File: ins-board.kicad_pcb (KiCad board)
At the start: 4 copper layers, 50 x 23 mm, 94 parts, among them P1 PWR, P2 Power (Solder Pad), Q1 FDN306P, Q2 FDC638APZ, U1 24LC128, U10 HMC5883L, U11 H3LIS331DL, U2 STM32F415RGT6, U3 LTC4412, U4 MAX3051, U5 LT1965, U6 LT1761-3.3, U7 LT1965, U8 MS5611-01BA, U9 MPU6000, X1 CRYSTAL 16MHz 10ppm

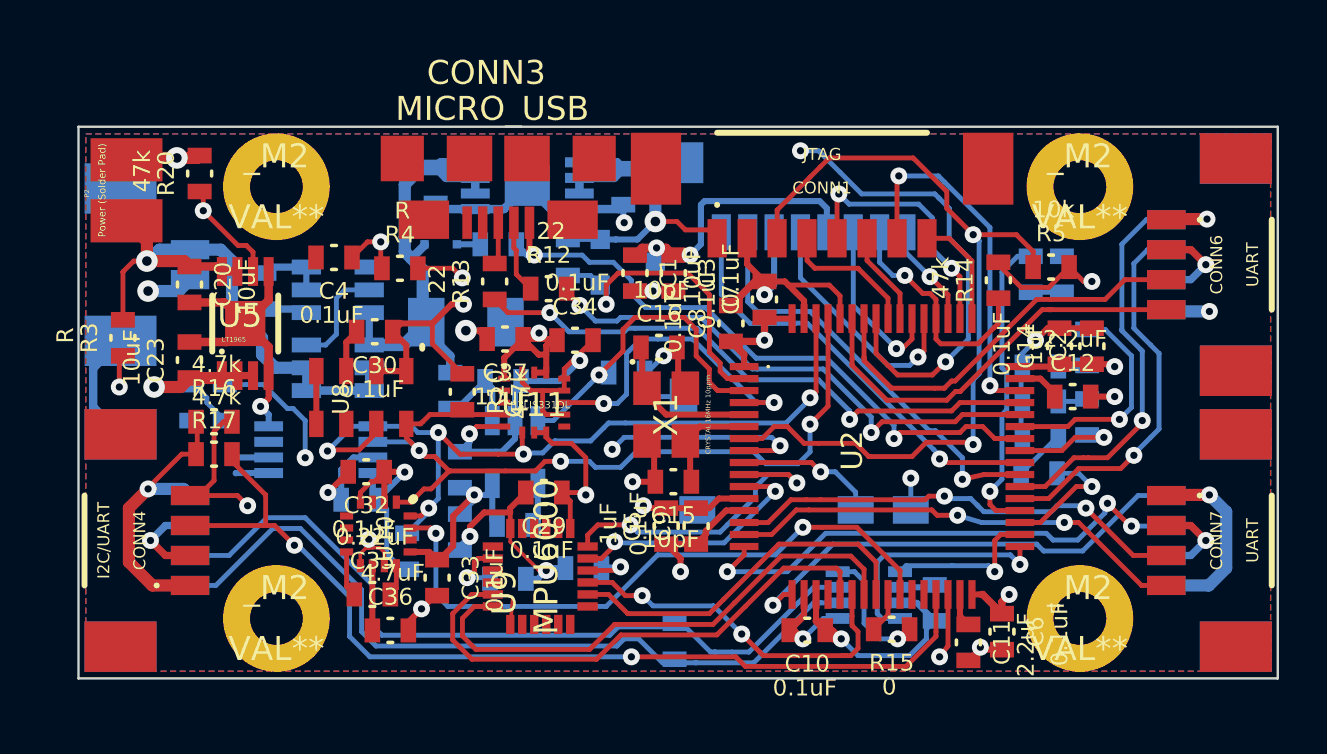
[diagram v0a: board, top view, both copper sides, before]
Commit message: optimize routing
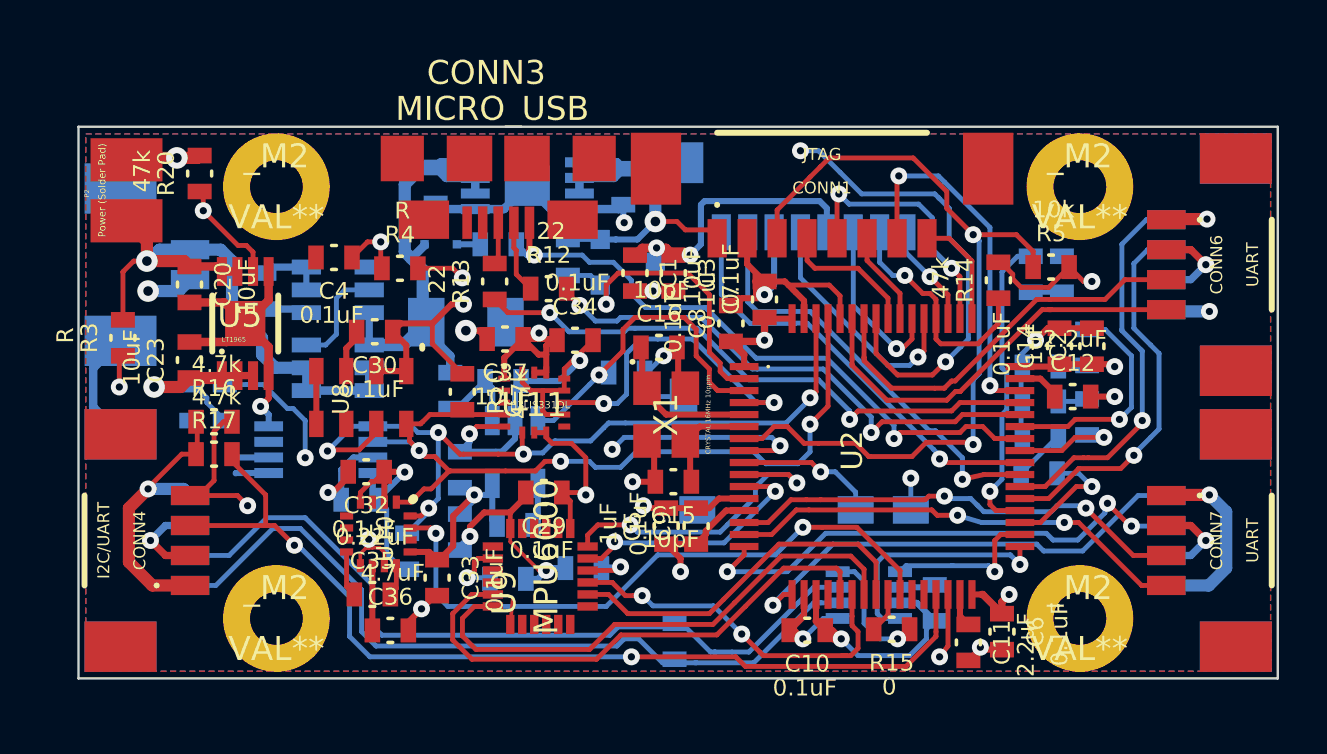
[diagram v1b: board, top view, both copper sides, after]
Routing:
- net GND: track 143.3 -> 144.7 mm
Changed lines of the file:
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@@
     (thickness 1.6)
     (drawings 13)
-    (tracks 1282)
+    (tracks 1293)
     (zones 0)
     (modules 94)
@@
   )
   (setup
-    (last_trace_width 0.2032)
+    (last_trace_width 0.254)
     (user_trace_width 0.1524)
     (user_trace_width 0.2032)
@@
   (segment (start 61.05 43.85) (end 56.15 43.85) (width 0.2032) (layer B.Cu) (net 27))
   (segment (start 62.2 42.7) (end 61.05 43.85) (width 0.2032) (layer B.Cu) (net 27))
-  (segment (start 45.6646 38.3872) (end 45.6646 38.9646) (width 0.2032) (layer F.Cu) (net 28))
-  (segment (start 45.6646 38.9646) (end 46.2 39.5) (width 0.2032) (layer F.Cu) (net 28))
+  (segment (start 45.6646 38.3872) (end 45.8 38.5226) (width 0.2032) (layer F.Cu) (net 28))
+  (segment (start 45.8 38.5226) (end 45.8 39.1) (width 0.2032) (layer F.Cu) (net 28))
+  (segment (start 45.8 39.1) (end 46.2 39.5) (width 0.2032) (layer F.Cu) (net 28))
   (segment (start 46.85 39.75) (end 46.45 39.75) (width 0.2032) (layer F.Cu) (net 28))
   (segment (start 46.45 39.75) (end 46.2 39.5) (width 0.2032) (layer F.Cu) (net 28))
@@
   (segment (start 66.25 38.75) (end 66 39) (width 0.2032) (layer F.Cu) (net 51))
   (segment (start 66.25 38.75) (end 66 39) (width 0.2032) (layer F.Cu) (net 51))
+  (segment (start 60.6 33) (end 60.45 33.15) (width 0.254) (layer F.Cu) (net 52))
+  (segment (start 59.5 33.15) (end 59.2 33.45) (width 0.254) (layer F.Cu) (net 52) (status C00000))
+  (segment (start 59.7 33.15) (end 59.5 33.15) (width 0.254) (layer F.Cu) (net 52) (status C00000))
+  (segment (start 60.45 33.15) (end 59.7 33.15) (width 0.254) (layer F.Cu) (net 52) (status 800000))
+  (segment (start 60.6 32.45) (end 60.25 32.8) (width 0.254) (layer F.Cu) (net 52) (status 400000))
+  (segment (start 60.25 32.8) (end 60.25 33) (width 0.254) (layer F.Cu) (net 52))
+  (segment (start 60.25 33) (end 60.6 33) (width 0.254) (layer F.Cu) (net 52))
+  (segment (start 50.65 41.25) (end 50.65 41.42) (width 0.254) (layer F.Cu) (net 52) (status C00000))
+  (segment (start 50.65 41.42) (end 49.99 42.08) (width 0.254) (layer F.Cu) (net 52) (status 400000))
+  (segment (start 43.2428 40.386) (end 43.2428 40.6072) (width 0.254) (layer F.Cu) (net 52))
+  (segment (start 42.6 41.25) (end 42.4 41.25) (width 0.254) (layer F.Cu) (net 52))
+  (segment (start 43.2428 40.6072) (end 42.6 41.25) (width 0.254) (layer F.Cu) (net 52))
+  (segment (start 43.5984 34.544) (end 43.5984 34.8016) (width 0.254) (layer F.Cu) (net 52))
+  (segment (start 43.5984 34.8016) (end 43.1646 35.2354) (width 0.254) (layer F.Cu) (net 52))
   (segment (start 79 43.25) (end 79.65 43.25) (width 0.508) (layer Inner2.Cu) (net 52))
   (segment (start 46.15 31.9) (end 47.6 31.9) (width 0.2032) (layer F.Cu) (net 52))
@@
   (via (at 39.59 37.66) (size 0.706) (layers F.Cu B.Cu) (net 52))
   (segment (start 39.925 37.325) (end 39.59 37.66) (width 0.254) (layer F.Cu) (net 52))
-  (segment (start 49.99 42.08) (end 49.99 41.91) (width 0.254) (layer F.Cu) (net 52))
-  (segment (start 49.99 41.91) (end 50.65 41.25) (width 0.254) (layer F.Cu) (net 52))
   (segment (start 47.9 43.65) (end 47.9 43.5) (width 0.254) (layer B.Cu) (net 52))
   (segment (start 48.91 42.08) (end 49.99 42.08) (width 0.254) (layer F.Cu) (net 52))
@@
   (segment (start 50 42.75) (end 50 42.08) (width 0.2032) (layer F.Cu) (net 52))
   (segment (start 47.9 39.55) (end 49.4 39.55) (width 0.254) (layer B.Cu) (net 52))
-  (segment (start 43.2428 40.386) (end 43.2428 40.4072) (width 0.254) (layer F.Cu) (net 52))
-  (segment (start 43.2428 40.4072) (end 42.4 41.25) (width 0.254) (layer F.Cu) (net 52))
   (segment (start 42.4 41.25) (end 42.65 41.25) (width 0.2032) (layer B.Cu) (net 52))
   (via (at 42.4 41.25) (size 0.706) (layers F.Cu B.Cu) (net 52))
@@
   (segment (start 42.95 40.3) (end 43.4632 39.7868) (width 0.254) (layer B.Cu) (net 52))
   (segment (start 41.9146 38.3872) (end 41.9146 36.1872) (width 0.254) (layer F.Cu) (net 52))
-  (segment (start 43.1646 36.1872) (end 43.1646 34.9778) (width 0.254) (layer F.Cu) (net 52))
-  (segment (start 43.1646 34.9778) (end 43.5984 34.544) (width 0.254) (layer F.Cu) (net 52))
+  (segment (start 43.1646 36.1872) (end 43.1646 35.2354) (width 0.254) (layer F.Cu) (net 52))
   (segment (start 66.7 41.975) (end 66.7 40.65) (width 0.2032) (layer B.Cu) (net 52))
   (via (at 66.7 40.65) (size 0.706) (layers F.Cu B.Cu) (net 52))
@@
   (via (at 55.1 40.8) (size 0.706) (layers F.Cu B.Cu) (net 52))
   (segment (start 61 30.4) (end 61 32.6) (width 0.254) (layer B.Cu) (net 52))
+  (segment (start 61 32.6) (end 60.6 33) (width 0.254) (layer B.Cu) (net 52))
   (via (at 60.6 33) (size 0.706) (layers F.Cu B.Cu) (net 52))
   (segment (start 60.6 33) (end 60.6 32.45) (width 0.254) (layer F.Cu) (net 52))
-  (segment (start 61 32.6) (end 60.6 33) (width 0.254) (layer B.Cu) (net 52))
   (segment (start 66.25 45.2) (end 67.6 45.2) (width 0.254) (layer B.Cu) (net 52))
   (segment (start 67.6 45.2) (end 67.7 45.1) (width 0.254) (layer B.Cu) (net 52))
@@
   (segment (start 61.6 32.6) (end 61.45 32.45) (width 0.254) (layer F.Cu) (net 52))
   (segment (start 61.45 32.45) (end 60.2 32.45) (width 0.254) (layer F.Cu) (net 52))
-  (segment (start 60.2 32.45) (end 59.2 33.45) (width 0.3048) (layer F.Cu) (net 52))
   (segment (start 77.35 31.125) (end 78.375 31.125) (width 0.3048) (layer F.Cu) (net 52))
   (segment (start 78.375 32.375) (end 77.35 32.375) (width 0.3048) (layer B.Cu) (net 52))
@@
   (via (at 54.6 44.35) (size 0.706) (layers F.Cu B.Cu) (net 76))
   (segment (start 54.45 44.5) (end 54.6 44.35) (width 0.2032) (layer F.Cu) (net 76))
+  (segment (start 70.35 31.65) (end 70.45 31.65) (width 0.2032) (layer F.Cu) (net 77) (status C00000))
+  (segment (start 70.95 32.15) (end 70.95 32.35) (width 0.2032) (layer F.Cu) (net 77))
+  (segment (start 70.45 31.65) (end 70.95 32.15) (width 0.2032) (layer F.Cu) (net 77) (status 400000))
   (segment (start 44.275 30.175) (end 45.6 28.85) (width 0.2032) (layer Inner2.Cu) (net 77))
   (segment (start 45.6 28.85) (end 54.05 28.85) (width 0.2032) (layer Inner2.Cu) (net 77))
@@
   (segment (start 63.44 46.99) (end 63.8 47.35) (width 0.254) (layer F.Cu) (net 77))
   (segment (start 63.1324 46.99) (end 63.44 46.99) (width 0.254) (layer F.Cu) (net 77))
-  (segment (start 70.35 31.65) (end 70.35 31.75) (width 0.2032) (layer F.Cu) (net 77))
   (segment (start 72.45 32.7) (end 73.3 31.85) (width 0.2032) (layer F.Cu) (net 77))
   (segment (start 71.3 32.7) (end 72.45 32.7) (width 0.2032) (layer F.Cu) (net 77))
-  (segment (start 70.35 31.75) (end 71.3 32.7) (width 0.2032) (layer F.Cu) (net 77))
+  (segment (start 70.95 32.35) (end 71.3 32.7) (width 0.2032) (layer F.Cu) (net 77))
   (segment (start 69.25 45.5) (end 69.65 45.5) (width 0.254) (layer F.Cu) (net 77))
   (segment (start 69.7 45.5) (end 70.5 46.3) (width 0.254) (layer F.Cu) (net 77))
